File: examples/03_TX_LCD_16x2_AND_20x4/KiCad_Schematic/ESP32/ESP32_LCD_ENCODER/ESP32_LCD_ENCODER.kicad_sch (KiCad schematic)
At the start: 4 parts, among them SW1 ENCODER, U1 ESP32-WROOM-32, U2 LCD16X2

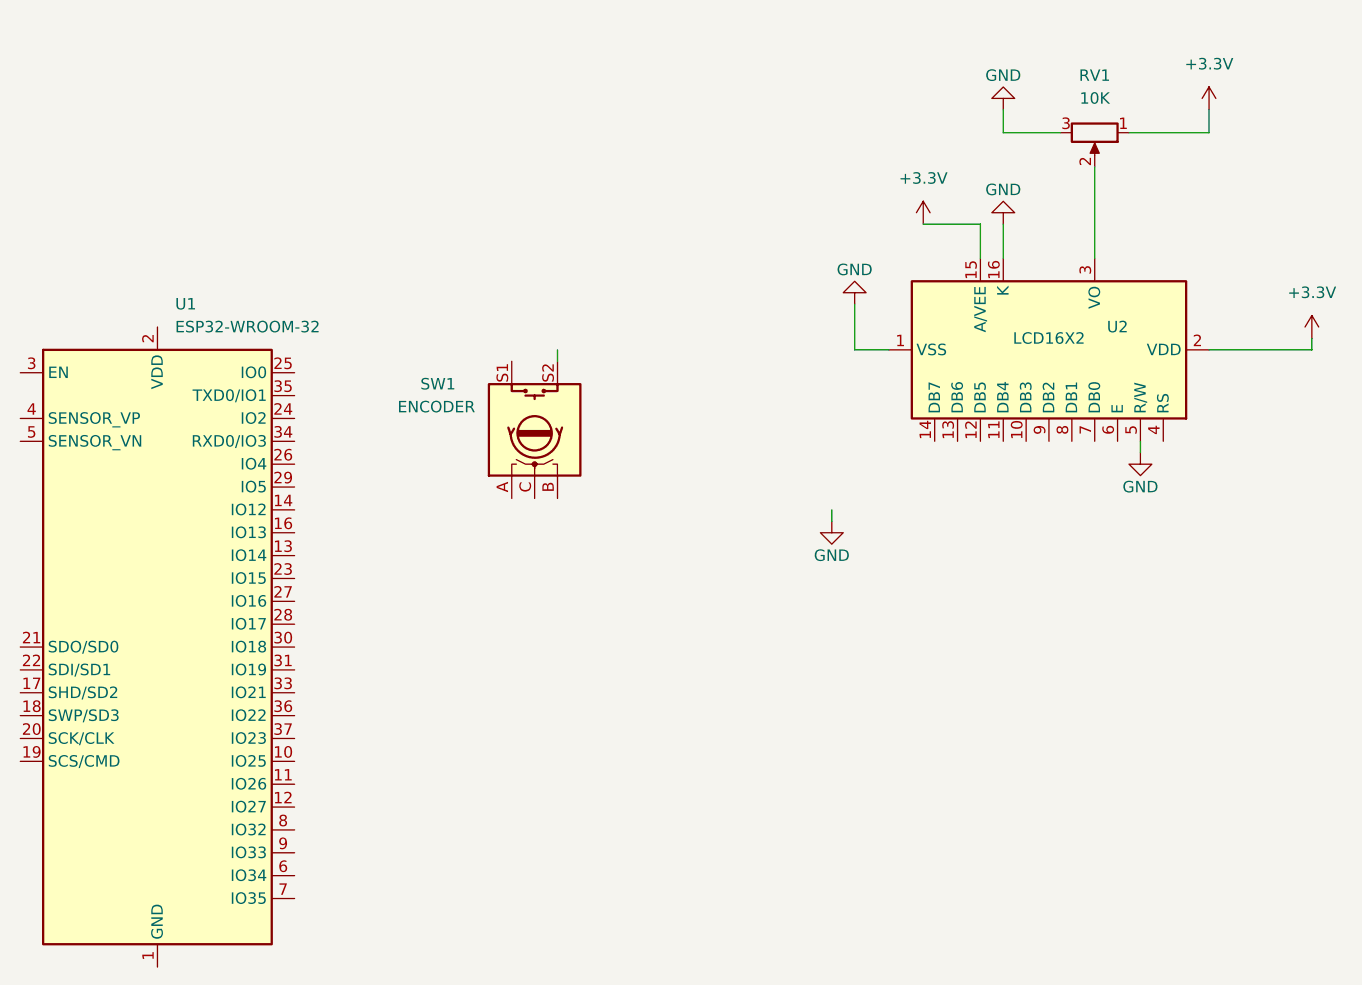
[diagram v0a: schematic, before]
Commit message: Doc
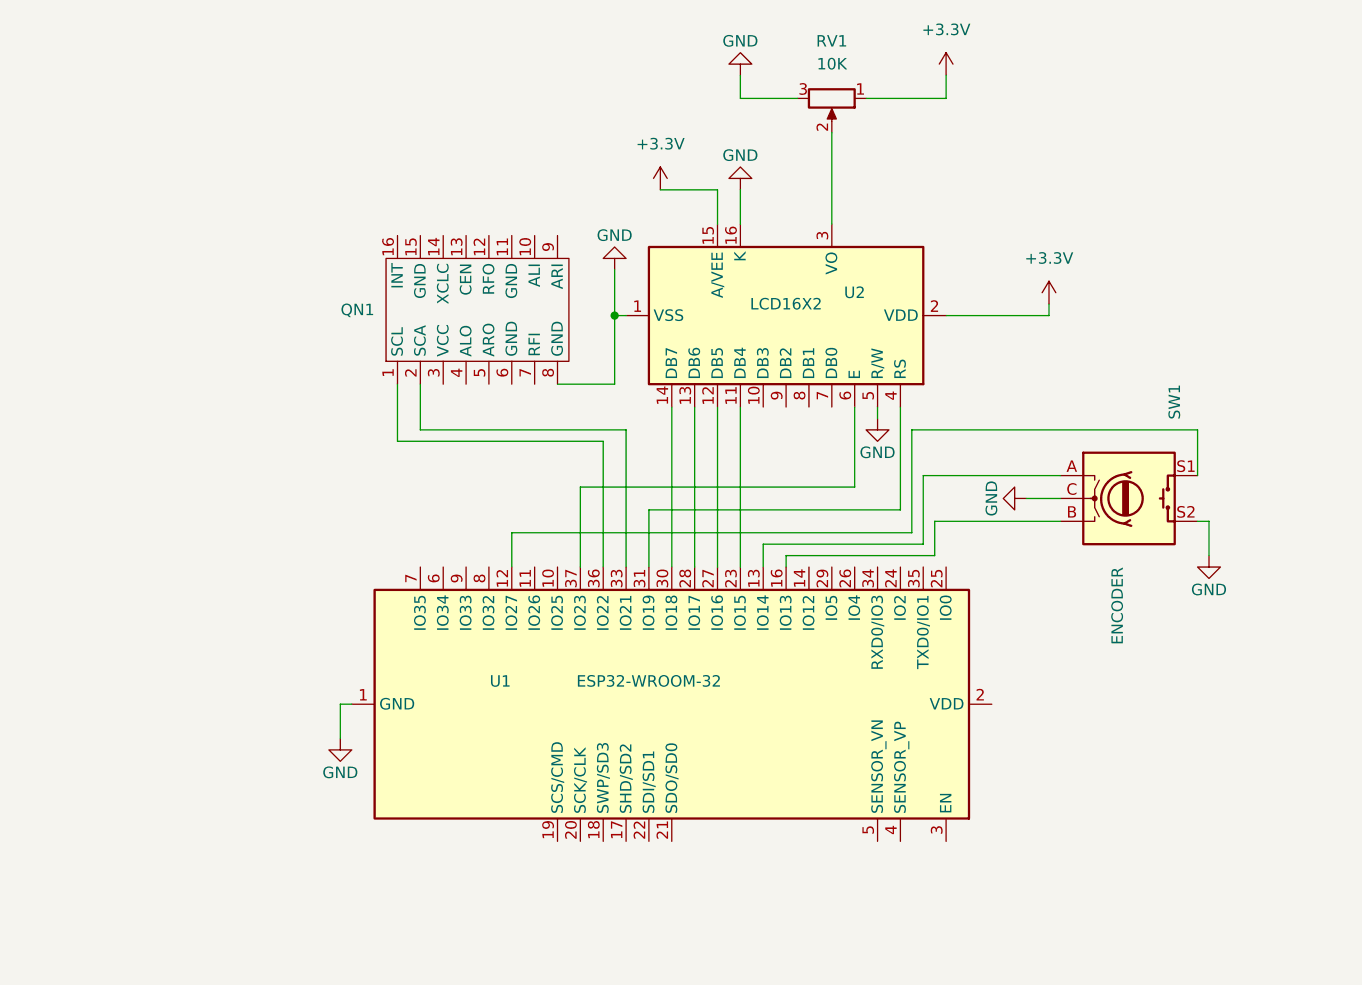
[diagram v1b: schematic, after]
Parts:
- added QN1: ~, symbol QN8066:QN8066
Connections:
- net GND: now also SW1.C, SW1.S2, U1.1 (GND), U1.15 (GND), U1.38 (GND), U1.39 (GND), QN1.8 (GND)
- net at U2.11 (DB4): now also U1.23 (IO15)
- net at U2.12 (DB5): now also U1.27 (IO16)
- net at U2.13 (DB6): now also U1.28 (IO17)
- net at U2.14 (DB7): now also U1.30 (IO18)
- net at U2.4 (RS): now also U1.31 (IO19)
- net at U2.6 (E): now also U1.37 (IO23)
- net at SW1.A: now also U1.13 (IO14)
- net at SW1.B: now also U1.16 (IO13)
- net at SW1.S1: now also U1.12 (IO27)
- net at U1.33 (IO21): now also QN1.2 (SCA)
- net at U1.36 (IO22): now also QN1.1 (SCL)
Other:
- moved on the sheet: RV1, SW1, U2
